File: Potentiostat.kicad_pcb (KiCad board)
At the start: 2 copper layers, 52 parts, among them IC1 LMP7702MA_NOPB, IC2 MAX4617ESE+, IC3 AMS1117-5.0, IC4 TEENSY3.2, IC5 LMP7702MA_NOPB, IC6 LMP7721MA_NOPB, SW1 KET_7X7

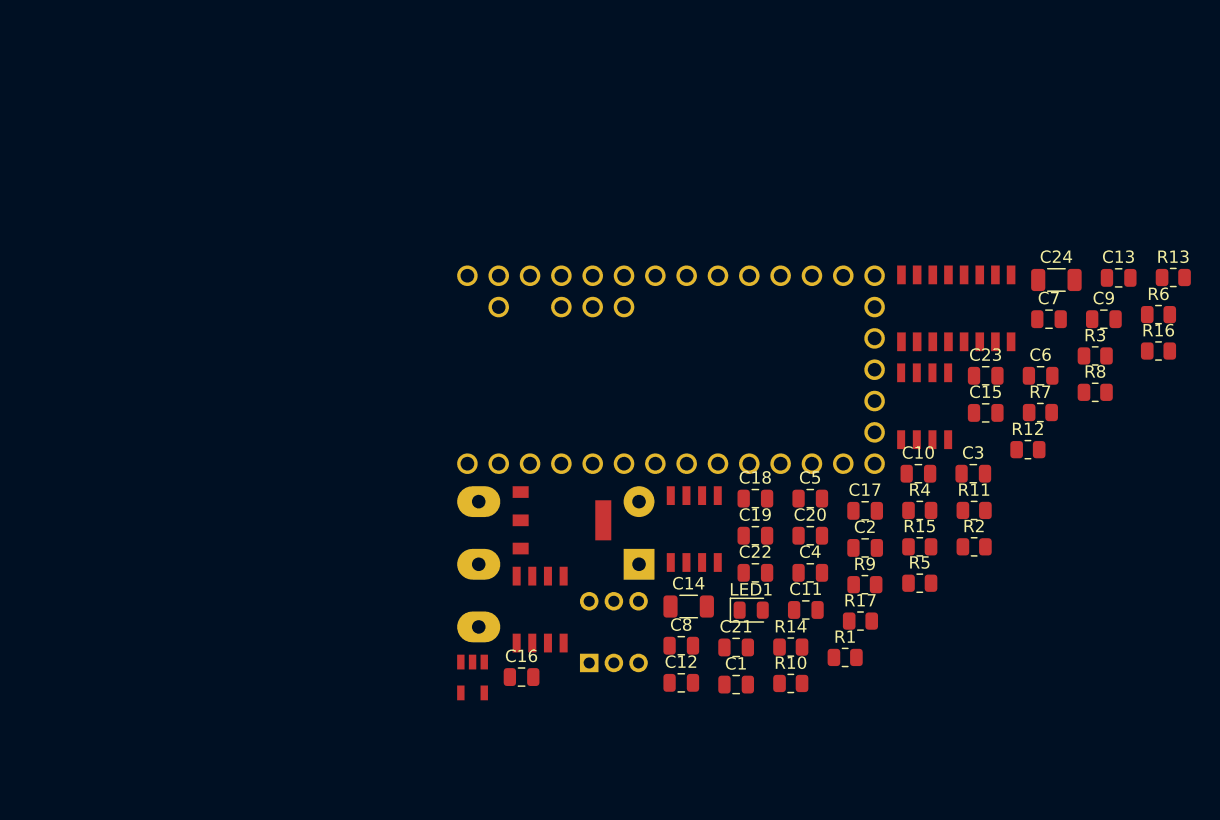
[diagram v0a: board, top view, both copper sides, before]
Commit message: Update Potentiostat.kicad_pcb
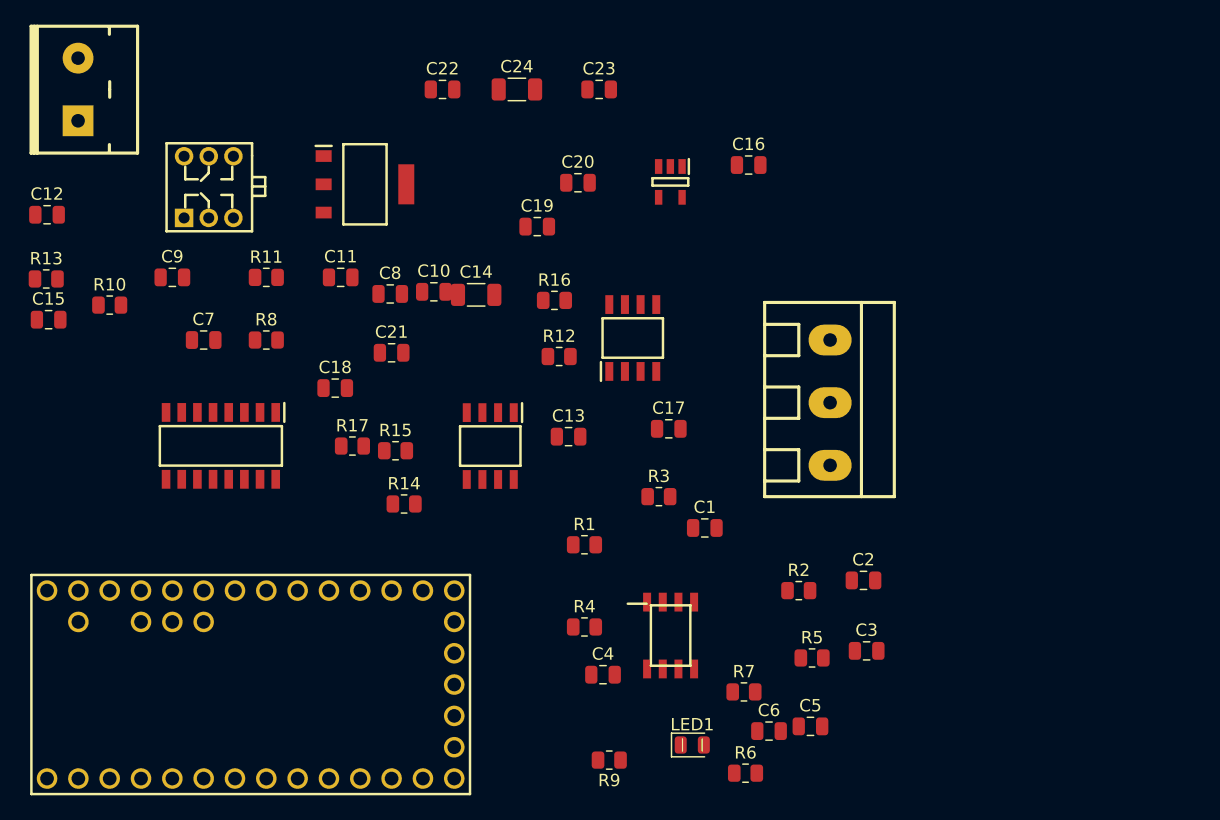
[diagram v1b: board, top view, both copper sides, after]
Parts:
- moved R13 91.4 mm to (101.5, 76.3)
- moved C15 76.4 mm to (101.7, 79.6)
- moved C9 75.6 mm to (111.8, 76.2)
- moved C7 68.6 mm to (114.3, 81.3)
- moved R8 67.4 mm to (119.4, 81.3)
- moved C12 63.9 mm to (101.6, 71.1)
- moved R10 63.2 mm to (106.7, 78.4)
- moved IC2 60.7 mm to (115.7, 89.9)
- moved R11 60.4 mm to (119.4, 76.2)
- moved JP1 58.0 mm to (104.1, 61.0)
- moved R6 50.0 mm to (158.2, 116.4)
- moved R16 49.2 mm to (142.7, 78.1)
- moved SW1 48.8 mm to (114.7, 68.9)
- moved C22 46.7 mm to (133.7, 61.0)
- moved C13 46.4 mm to (143.9, 89.1)
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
